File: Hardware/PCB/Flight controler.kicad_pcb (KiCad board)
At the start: 2 copper layers, 40 x 47.7 mm, 79 parts, among them J1 Screw_Terminal_01x02, J2 Conn_01x03, J3 Conn_01x03, SW1 TS-1088-AR02016, SW2 TS-1088-AR02016, U1 STM32F722RETx, U2 BQ25883RGER, U3 ICM-45686, U4 BMP580, U5 TPS63070RNMR, U6 LMR51430, X1 X322525MOB4SI, X2 Q13FC1350000400

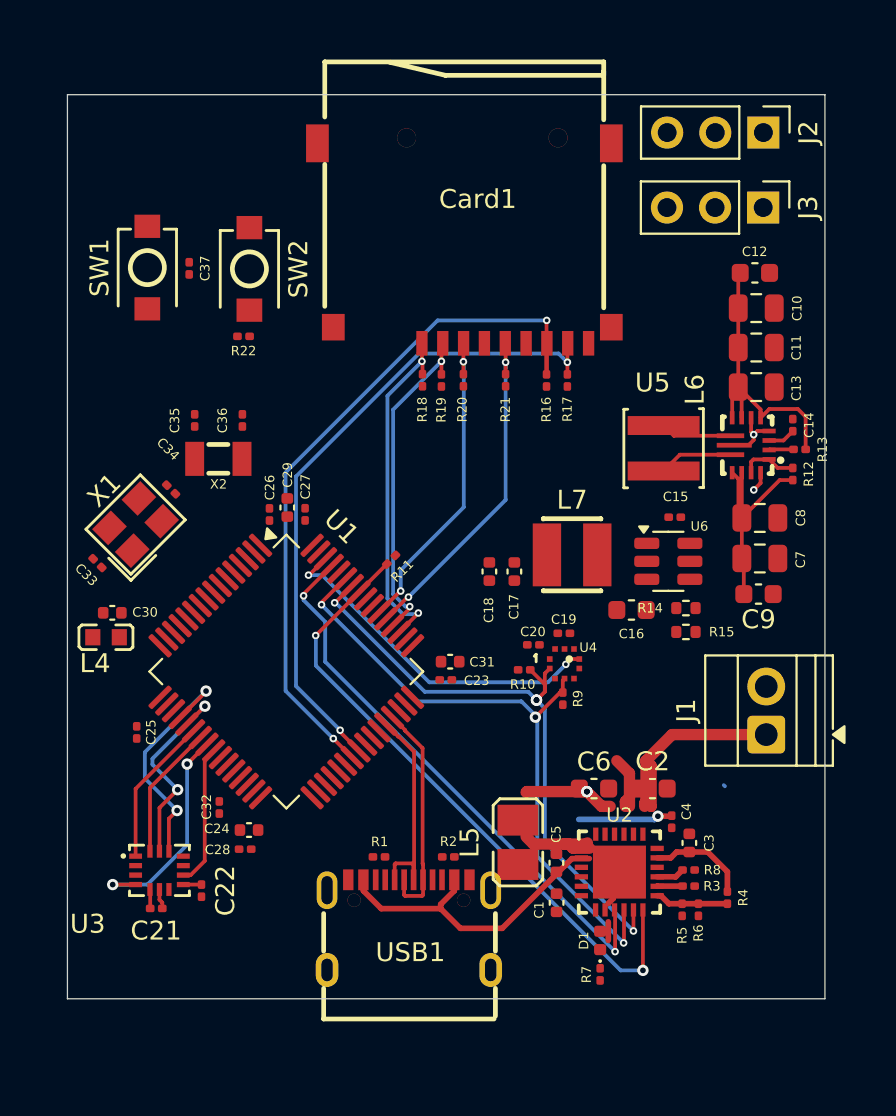
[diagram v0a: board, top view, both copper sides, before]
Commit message: Add files via upload
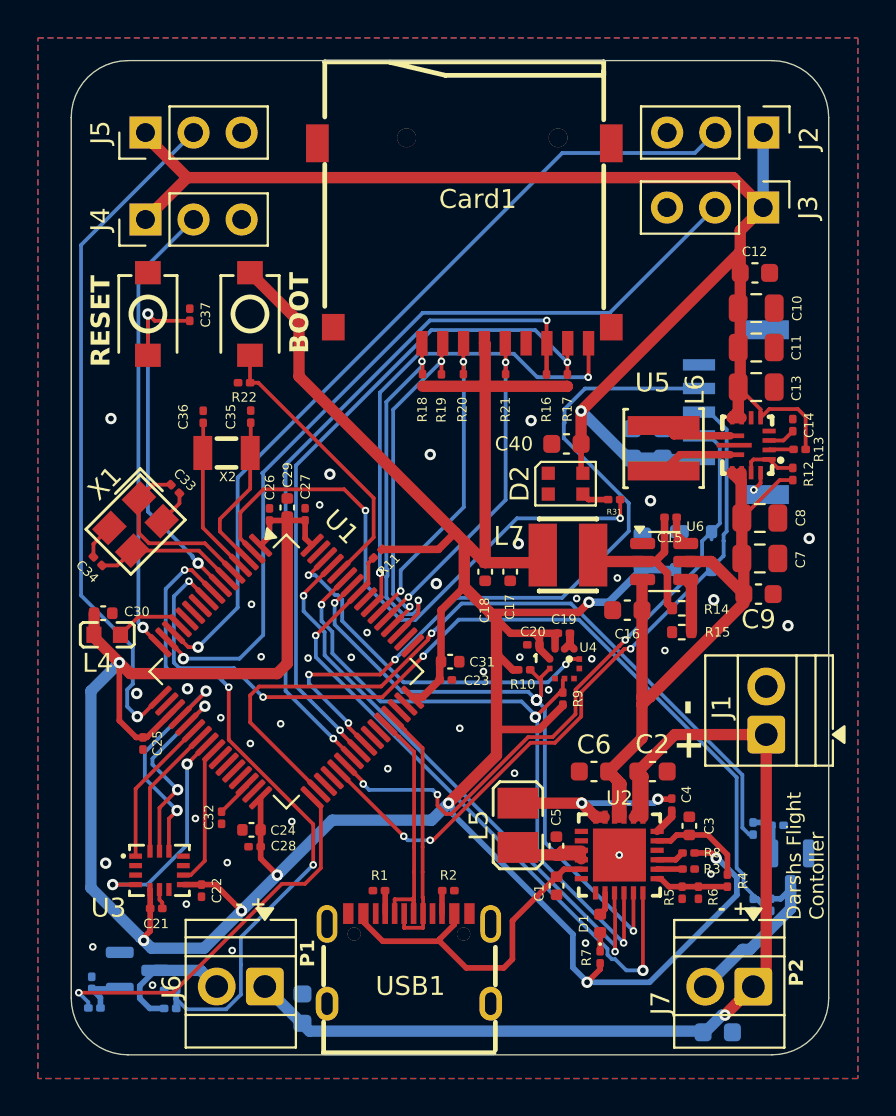
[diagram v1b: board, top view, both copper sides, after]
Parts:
- added C38: 10uF, Capacitor_SMD:C_0603_1608Metric, B.Cu at (150.4, 76.4)
- added C39: 100nf, Capacitor_SMD:C_0603_1608Metric, B.Cu at (152.0, 76.4)
- added C40: 100nf, Capacitor_SMD:C_0603_1608Metric, F.Cu at (147.0, 76.5)
- added C41: 100nf, Capacitor_SMD:C_0603_1608Metric, B.Cu at (151.0, 82.1)
- added C45: 100nf, Capacitor_SMD:C_0603_1608Metric, B.Cu at (154.9, 107.5)
- added C46: 100nf, Capacitor_SMD:C_0603_1608Metric, B.Cu at (133.0, 106.3)
- added D2: WS2812B-2020, LED_SMD:LED_WS2812B-2020_PLCC4_2.0x2.0mm, F.Cu at (146.9, 78.5)
- added D3: PRTR5V0U2X, Package_TO_SOT_SMD:SOT-143, B.Cu at (153.7, 82.1)
- added J4: Conn_01x03, Connector_PinHeader_2.54mm:PinHeader_1x03_P2.54mm_Vertical, F.Cu at (124.7, 64.6)
- added J5: Conn_01x03, Connector_PinHeader_2.54mm:PinHeader_1x03_P2.54mm_Vertical, F.Cu at (124.7, 60.0)
- added J6: Screw_Terminal_01x02, TerminalBlock:TerminalBlock_Xinya_XY308-2.54-2P_1x02_P2.54mm_Horizontal, F.Cu at (131.0, 105.1)
- added J7: Screw_Terminal_01x02, TerminalBlock:TerminalBlock_Xinya_XY308-2.54-2P_1x02_P2.54mm_Horizontal, F.Cu at (156.8, 105.1)
- added J8: BM05B-GHS-TBT_LF__SN__N_, BM05B-GHS-TBT_LF__SN__N_:JST_BM05B-GHS-TBT_LF__SN__N_, B.Cu at (156.3, 74.8)
- added Q1: AO3400A, Package_TO_SOT_SMD:SOT-23, B.Cu at (124.3, 104.2)
- added Q2: AO3400A, Package_TO_SOT_SMD:SOT-23, B.Cu at (158.8, 99.0)
- added R23: 10K, Resistor_SMD:R_0201_0603Metric, B.Cu at (121.9, 104.9)
- added R24: 100K, Resistor_SMD:R_0201_0603Metric, B.Cu at (126.0, 106.3)
- added R25: 100, Resistor_SMD:R_0201_0603Metric, B.Cu at (122.0, 106.2)
- added R26: 10K, Resistor_SMD:R_0201_0603Metric, B.Cu at (126.0, 105.3)
- added R27: 100, Resistor_SMD:R_0201_0603Metric, B.Cu at (156.8, 96.8)
- added R28: 10K, Resistor_SMD:R_0201_0603Metric, B.Cu at (158.1, 96.6)
- added R29: 100K, Resistor_SMD:R_0201_0603Metric, B.Cu at (157.7, 100.8)
- added R30: 10K, Resistor_SMD:R_0201_0603Metric, B.Cu at (156.8, 100.8)
- added R31: 100, Resistor_SMD:R_0201_0603Metric, F.Cu at (149.5, 79.4)
- R3: value 383 -> .383k
- moved C33 5.67 mm to (126.3, 78.8), turned to -45 degrees
- moved C34 5.42 mm to (122.2, 82.6), turned to 135 degrees
- moved C35 2.97 mm to (130.3, 75.0)
- moved R22 2.45 mm to (129.9, 73.2)
- moved RESET 2.45 mm to (124.9, 69.6)
- moved C37 2.45 mm to (127.1, 69.6)
- moved BOOT 2.38 mm to (130.2, 69.6)
- moved C36 2.08 mm to (127.8, 75.0)
- moved R1 1.78 mm to (137.1, 100.0)
- moved R2 1.78 mm to (140.7, 100.0)
- moved USB1 1.78 mm to (138.6, 103.6)
- moved C1 0.90 mm to (146.4, 99.8)
- moved C2 0.90 mm to (151.5, 93.8)
- moved C4 0.90 mm to (152.5, 95.5)
- moved C6 0.90 mm to (148.4, 93.8)
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- renumbered SW2 to BOOT, SW1 to RESET
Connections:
- U1 pad 16: unconnected-(U1-PA2-Pad16) -> /SERVO3
- U1 pad 17: unconnected-(U1-PA3-Pad17) -> /SERVO4
- U1 pad 2: unconnected-(U1-PC13-Pad2) -> /STATUS_LED
- U1 pad 33: unconnected-(U1-PB12-Pad33) -> /PYRO_1
- U1 pad 34: unconnected-(U1-PB13-Pad34) -> /PYRO_2
- U1 pad 37: unconnected-(U1-PC6-Pad37) -> /USART6_TX
- U1 pad 38: unconnected-(U1-PC7-Pad38) -> /USART6_RX
- U1 pad 41: unconnected-(U1-PA8-Pad41) -> /PPS
- U1 pad 8: unconnected-(U1-PC0-Pad8) -> /PYRO_CON_1
- U1 pad 9: unconnected-(U1-PC1-Pad9) -> /PYRO_CON_2
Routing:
- net +3.3V: track 1.96 -> 199.0 mm, vias 0 -> 8
- net +5V: track 16.1 -> 90.6 mm, vias 0 -> 1
- net /PYRO_CON_2: track 0.00 -> 50.1 mm, vias 0 -> 3
- net /SERVO2: track 0.00 -> 44.4 mm, vias 0 -> 1
- net /SERVO1: track 0.00 -> 44.2 mm, vias 0 -> 1
- net /PYRO_2: track 0.00 -> 41.9 mm, vias 0 -> 1
- net /PPS: track 0.00 -> 40.4 mm, vias 0 -> 3
- net BAT+: track 15.5 -> 53.9 mm, vias 0 -> 1
- net /USART6_TX: track 0.00 -> 37.4 mm, vias 0 -> 3
- net /SERVO4: track 0.00 -> 36.4 mm, vias 0 -> 1
- net /PYRO_CON_1: track 0.00 -> 35.9 mm, vias 0 -> 3
- net /USART6_RX: track 0.00 -> 35.2 mm, vias 0 -> 3
- net /STATUS_LED: track 0.00 -> 31.3 mm, vias 0 -> 2
- net VSYS: track 12.6 -> 39.1 mm
- net /SD_CD: track 0.00 -> 25.6 mm, vias 0 -> 3
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- added copper zone on B.Cu, net GND
- added copper zone on F.Cu, net GND
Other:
- board size 40 x 47.7 mm -> 40 x 52.5 mm
- board text added: "+ -"
- board text added: "Darshs Flight Contoller"
- board text added: "P1"
- board text added: "P2"
